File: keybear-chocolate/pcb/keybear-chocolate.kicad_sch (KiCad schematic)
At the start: 102 parts, among them J1 MJ-4PP-9, J2 BATT, J3 LED, J4 OLED, SW1 SW_PUSH, SW10 SW_PUSH, SW11 SW_PUSH, SW12 SW_PUSH, SW13 SW_PUSH, SW14 SW_PUSH, SW15 SW_PUSH, SW16 SW_PUSH, SW17 SW_PUSH, SW18 SW_PUSH, SW19 SW_PUSH, SW2 SW_PUSH, SW20 SW_PUSH, SW21 SW_PUSH, SW22 SW_PUSH, SW25 Rotary_Encoder_Switch, SW3 SW_PUSH, SW30 BATT_SW, SW4 SW_PUSH, SW5 SW_PUSH, SW6 SW_PUSH, SW7 SW_PUSH, SW8 SW_PUSH, SW9 SW_PUSH, U1 ProMicro

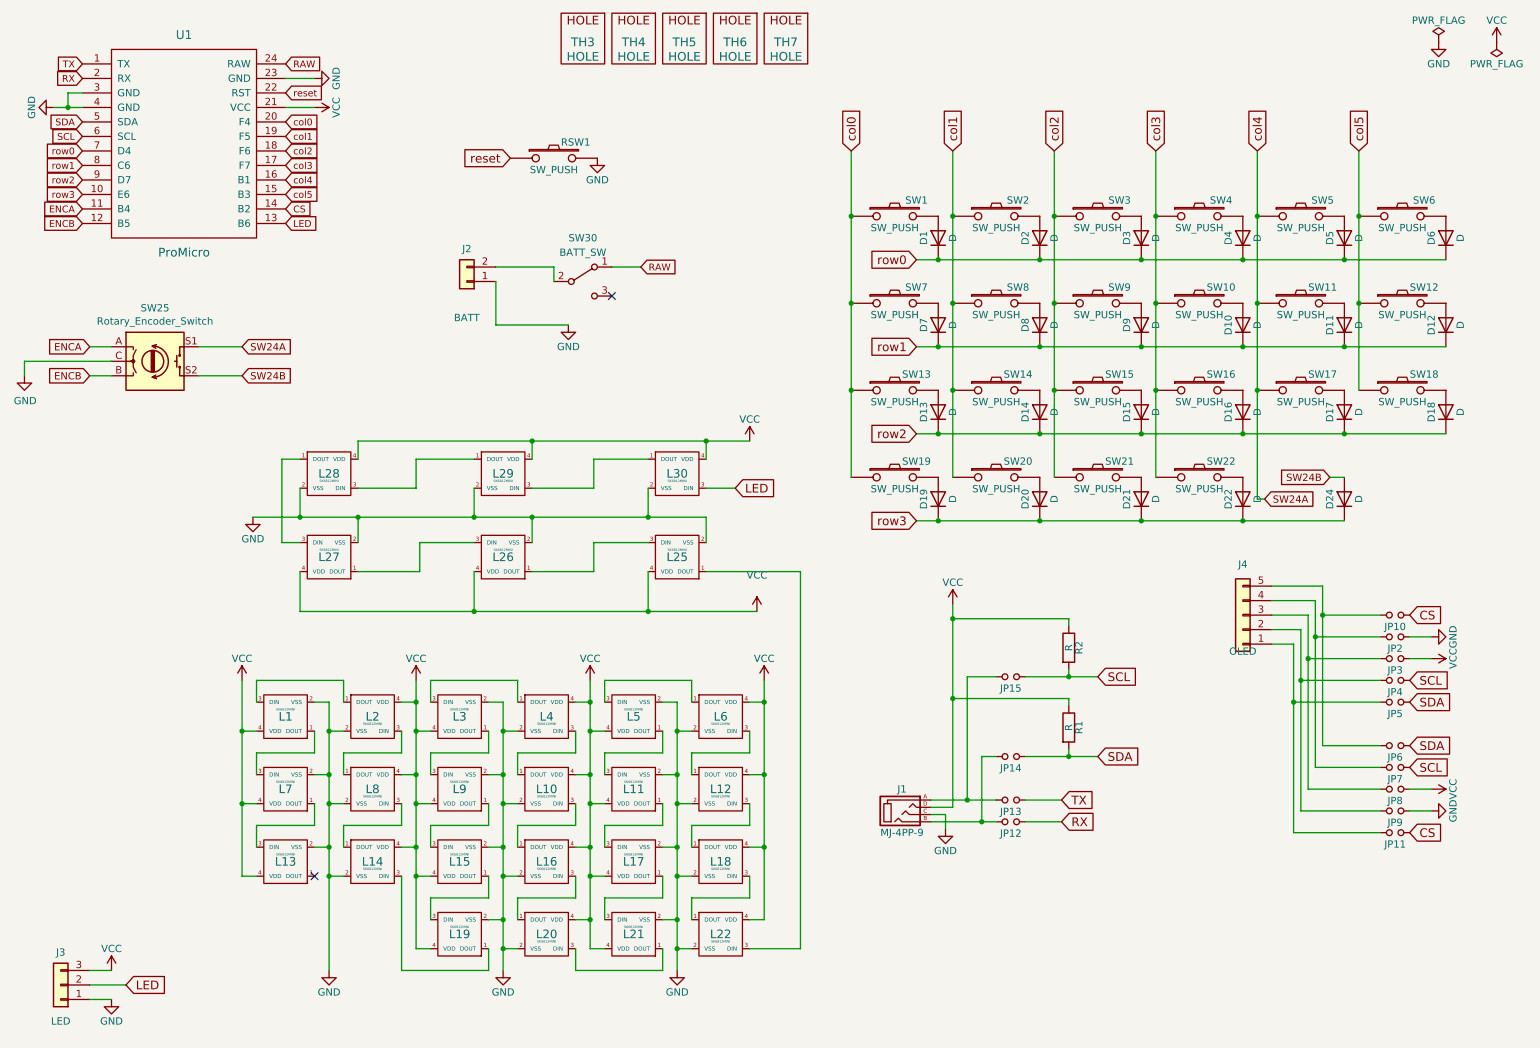
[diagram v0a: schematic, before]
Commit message: usb-c added - WIP
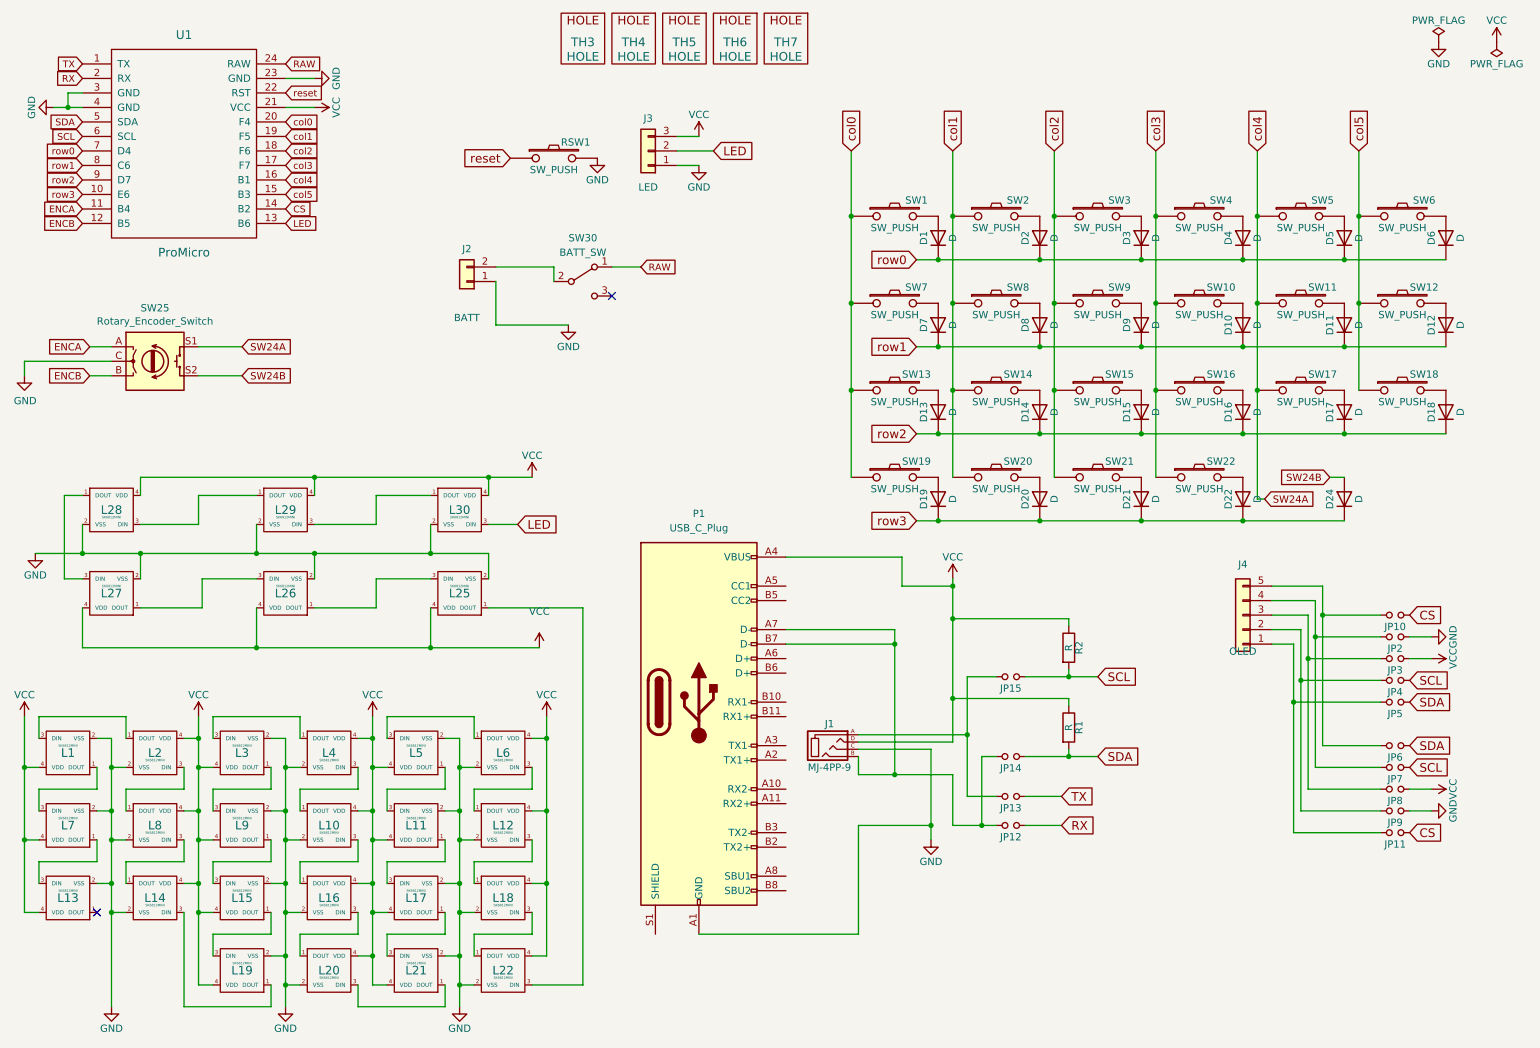
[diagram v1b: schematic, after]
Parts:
- added P1: USB_C_Plug, Connector_USB:USB_C_Receptacle_G-Switch_GT-USB-7010ASV, symbol Connector:USB_C_Receptacle
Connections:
- net GND: now also P1.A1 (GND), P1.A12 (GND), P1.B1 (GND), P1.B12 (GND)
- net VCC: now also P1.A4 (VBUS), P1.A9 (VBUS), P1.B4 (VBUS), P1.B9 (VBUS)
- net at J1.B, JP12.2, JP14.2: now also P1.A7 (D-), P1.B7 (D-)
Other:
- moved on the sheet: J1, J3, JP12, JP13, L1, L10, L11, L12, L13, L14, L15, L16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
